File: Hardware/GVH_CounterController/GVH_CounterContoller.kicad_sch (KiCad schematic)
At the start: 37 parts, among them J1 Molex Ultra-Fit, J2 Barrel jack, J3 WIZnet_J1B1211CCD_RJ45, K1 Relay_DPDT, Q1 MBT2222, SW1 SW_DIP_x02, SW2 SW_MEC_5G, U1 Teensy4.1, U2 R-78E5.0-1.0, U3 RT9080-3.3, U4 DS18B20_

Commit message: Added Mosfet fan controller to CounterController Schematic
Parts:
- removed J2: Barrel jack, Connector_BarrelJack:BarrelJack_Horizontal, symbol Connector:Barrel_Jack_Switch
- added C16: 0.1uF, Capacitor_SMD:C_0402_1005Metric, symbol Device:C_Small
- added D7, D8: PMEG10030, Diode_SMD:D_SOD-128, symbol Device:D
- added J10, J11, J12, J2, J8, J9: Molex Micro-Fit 2pos, 0_connector:MOLEX_MICROFIT-VERT-2POS_436500215, symbol 0_connector:Molex Micro-Fit 2pos
- added J13: Molex Micro-Fit 3pos, 0_connector:MOLEX_MICROFIT-VERT-3POS_436500315, symbol 0_connector:Molex Micro-Fit 3pos Vert
- added JP2: SolderJumper_2_Bridged, Jumper:SolderJumper-2_P1.3mm_Bridged_RoundedPad1.0x1.5mm, symbol Jumper:SolderJumper_2_Bridged
- added Q2, Q3: AO3406, Package_TO_SOT_SMD:SOT-23, symbol Transistor_FET:AO3400A
- added R10, R8: 100R, Resistor_SMD:R_0603_1608Metric, symbol Device:R_Small
- added R11, R12: 10k, Resistor_SMD:R_0603_1608Metric, symbol Device:R_Small
- added R9: 4.7k, Resistor_SMD:R_0603_1608Metric, symbol Device:R
- added U14: SN74LVC2G17, Package_TO_SOT_SMD:SOT-23-6, symbol 0_integrated_circuits:SN74LVC2G17
- D1: Package (none) -> TO-277
- JP1: now left out of the parts list
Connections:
- net +12V: now also D7.1 (K), D8.1 (K), J10.2 (Pin_2), J11.2 (Pin_2), J12.2 (Pin_2), J2.2 (Pin_2), J8.2 (Pin_2), J9.2 (Pin_2)
- net +3.3V: now also J13.2 (Pin_2), JP2.1 (A), R9.2; no longer D5.2 (A)
- net +5V: now also C16.1, U14.5 (VCC)
- net GND: now also C16.2, J13.1 (Pin_1), Q2.2 (S), Q3.2 (S), R11.1, R12.1, U14.2 (GND)
- net IO_Level_Shift2/CLK: no longer U1.33 (41_A17)
- net IO_Level_Shift2/LOAD: no longer U1.32 (40_A16)
- net IO_Level_Shift2/SERIAL_IN: no longer U1.31 (39_MISO1_OUT1A)
- net IO_Level_Shift3/CLK: no longer U1.27 (35_TX8)
- net IO_Level_Shift3/LOAD: no longer U1.26 (34_RX8)
- net IO_Level_Shift3/SERIAL_IN: no longer U1.25 (33_MCLK2)
- net SER_0: now reaches U1.12 (10_CS_MQSR)
- net CLK_0: now reaches U1.13 (11_MOSI_CTX1)
- net LOAD_0: now reaches U1.14 (12_MISO_MQSL)
- net SER_1: now reaches U1.20 (28_RX7)
- net CLK_1: now reaches U1.21 (29_TX7)
- net LOAD_1: now reaches U1.22 (30_CRX3)
- net DIP1 renamed DIP_0
- net DIP2 renamed DIP_1
- net IO_Level_Shift/CLK: no longer names the net of U1.45 (23_A9_CRX1_MCLK1)
- net IO_Level_Shift/LOAD: no longer names the net of U1.44 (22_A8_CTX1)
- net IO_Level_Shift/SERIAL_IN: no longer names the net of U1.43 (21_A7_RX5_BCLK1)
- net IO_Level_Shift1/CLK: no longer names the net of U1.39 (17_A3_TX4_SDA1)
- net IO_Level_Shift1/LOAD: no longer names the net of U1.38 (16_A2_RX4_SCL1)
- net IO_Level_Shift1/SERIAL_IN: no longer names the net of U1.37 (15_A1_RX3_SPDIF_IN)
- net TEMP_SENS1 renamed TEMP_SENS_0
- new net: Q2.1 (G), R8.2
- new net: D7.2 (A), J11.1 (Pin_1), J12.1 (Pin_1), Q2.3 (D)
- new net: R10.1, R11.2, U14.4 (2Y)
- new net: R12.2, R8.1, U14.6 (1Y)
- new net: D8.2 (A), J10.1 (Pin_1), J2.1 (Pin_1), J8.1 (Pin_1), J9.1 (Pin_1), Q3.3 (D)
- new net: D5.2 (A), JP2.2 (B)
- new net: Q3.1 (G), R10.2
- new net FAN_0: U14.1 (1A)
- new net FAN_1: U14.3 (2A)
- new net TEMP_SENS_1: J13.3 (Pin_3), R9.1
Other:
- note added: "RED LED"
- note removed: "3.3V RED LED"
- moved on the sheet: D5, D6, R6, R7, U4

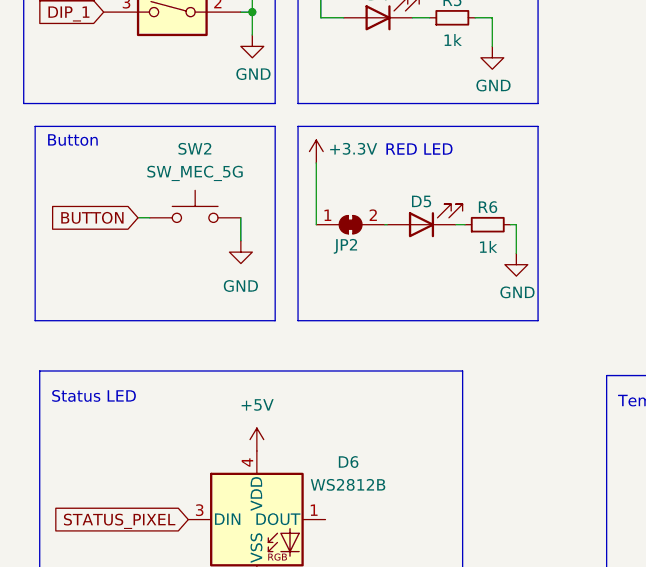
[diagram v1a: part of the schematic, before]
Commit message: Checkpoint before rerouting the power supply
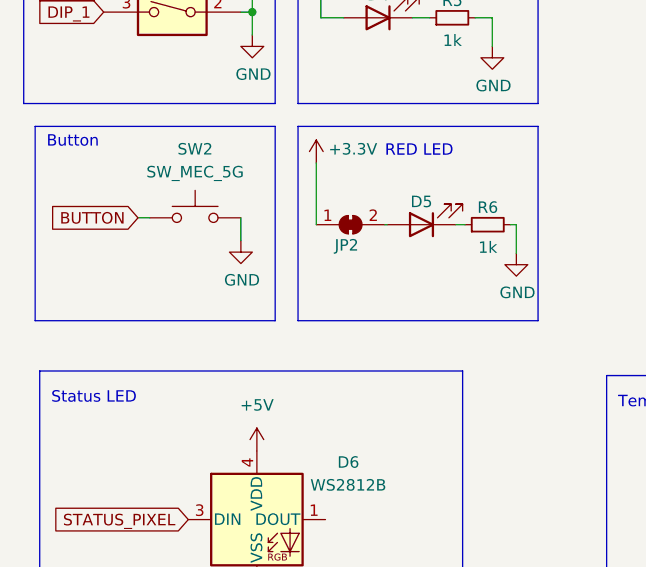
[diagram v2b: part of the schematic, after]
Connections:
- net BUTTON: no longer SW2.2 (B)
- net GND: no longer SW2.4 (B)
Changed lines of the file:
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@@
       (effects (font (size 1.27 1.27)) hide)
     )
-    (property "Datasheet" "" (at 53.34 172.72 0)
+    (property "Datasheet" "https://omronfs.omron.com/en_US/ecb/products/pdf/en-b3f.pdf" (at 53.34 172.72 0)
       (effects (font (size 1.27 1.27)) hide)
     )
@@
       (effects (font (size 1.27 1.27)) hide)
     )
-    (property "Manufacturer" "Omron Electronics Inc-EMC Div" (at 53.34 177.8 0)
-      (effects (font (size 1.27 1.27)) hide)
-    )
-    (property "Digikey P/N" "SW402-ND" (at 53.34 177.8 0)
-      (effects (font (size 1.27 1.27)) hide)
-    )
-    (property "Digikey Page" "https://www.digikey.com/en/products/detail/omron-electronics-inc-emc-div/B3F-1020/44059" (at 53.34 177.8 0)
-      (effects (font (size 1.27 1.27)) hide)
-    )
-    (property "MPN" "B3F-1020" (at 53.34 177.8 0)
-      (effects (font (size 1.27 1.27)) hide)
-    )
-    (property "Description" "Tactile Switch SPST-NO Top Actuated Through Hole" (at 53.34 177.8 0)
-      (effects (font (size 1.27 1.27)) hide)
-    )
-    (pin "2")
-    (pin "4")
+    (property "Manufacturer" "Omron Electronics Inc-EMC Div" (at 53.086 182.88 0)
+      (effects (font (size 1.27 1.27)) hide)
+    )
+    (property "Digikey P/N" "SW402-ND" (at 52.324 186.944 0)
+      (effects (font (size 1.27 1.27)) hide)
+    )
+    (property "Digikey Page" "https://www.digikey.com/en/products/detail/omron-electronics-inc-emc-div/B3F-1020/44059" (at 53.34 180.594 0)
+      (effects (font (size 1.27 1.27)) hide)
+    )
+    (property "MPN" "B3F-1020" (at 53.086 179.324 0)
+      (effects (font (size 1.27 1.27)) hide)
+    )
+    (property "Description" "Tactile Switch SPST-NO Top Actuated Through Hole" (at 53.086 184.658 0)
+      (effects (font (size 1.27 1.27)) hide)
+    )
     (pin "1")
     (pin "2")
@@
     )
   )
+  (symbol (lib_id "power:GND") (at 58.42 180.34 0) (unit 1)
+    (in_bom yes) (on_board yes) (dnp no)
+    (property "Reference" "#PWR021" (at 58.42 186.69 0)
+      (effects (font (size 1.27 1.27)) hide)
+    )
+    (property "Value" "GND" (at 58.547 184.7342 0)
+      (effects (font (size 1.27 1.27)))
+    )
+    (property "Footprint" "" (at 58.42 180.34 0)
+      (effects (font (size 1.27 1.27)) hide)
+    )
+    (property "Datasheet" "" (at 58.42 180.34 0)
+      (effects (font (size 1.27 1.27)) hide)
+    )
+    (pin "1")
+    (instances
+      (project "GVH_CounterContoller"
+        (path "/2012002c-7ba5-4575-b93c-d8b37d21ac31"
+          (reference "#PWR021") (unit 1)
+        )
+      )
+      (project "KTX-MultiPCB"
+        (path "/aa56e0db-dcb9-4815-a5d6-811d95d9cf15/00000000-0000-0000-0000-00006034b2d9"
+          (reference "#PWR?") (unit 1)
+        )
+        (path "/aa56e0db-dcb9-4815-a5d6-811d95d9cf15"
+          (reference "#PWR04") (unit 1)
+        )
+      )
+    )
+  )
   (symbol (lib_id "Device:R_Small") (at 295.91 74.93 90) (unit 1)
     (in_bom yes) (on_board yes) (dnp no)
@@
         )
       )
-    )
-  )
-  (symbol (lib_id "power:GND") (at 58.42 180.34 0) (unit 1)
-    (in_bom yes) (on_board yes) (dnp no) (fields_autoplaced)
-    (property "Reference" "#PWR021" (at 58.42 186.69 0)
-      (effects (font (size 1.27 1.27)) hide)
-    )
-    (property "Value" "GND" (at 58.42 185.42 0)
-      (effects (font (size 1.27 1.27)))
-    )
-    (property "Footprint" "" (at 58.42 180.34 0)
-      (effects (font (size 1.27 1.27)) hide)
-    )
-    (property "Datasheet" "" (at 58.42 180.34 0)
-      (effects (font (size 1.27 1.27)) hide)
-    )
-    (pin "1")
-    (instances
-      (project "GVH_CounterContoller"
-        (path "/2012002c-7ba5-4575-b93c-d8b37d21ac31"
-          (reference "#PWR021") (unit 1)
-        )
-      )
-      (project "GVH-SwissArmyPCB"
-        (path "/38ccbc2b-e79d-43d1-80a7-cb797d9e77eb"
-          (reference "#PWR011") (unit 1)
-        )
-      )
